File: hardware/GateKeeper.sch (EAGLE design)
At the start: 26 parts, among them K1 G3VM-351A, K2 G3VM-351A, U1 WEMOS-C3-PICO

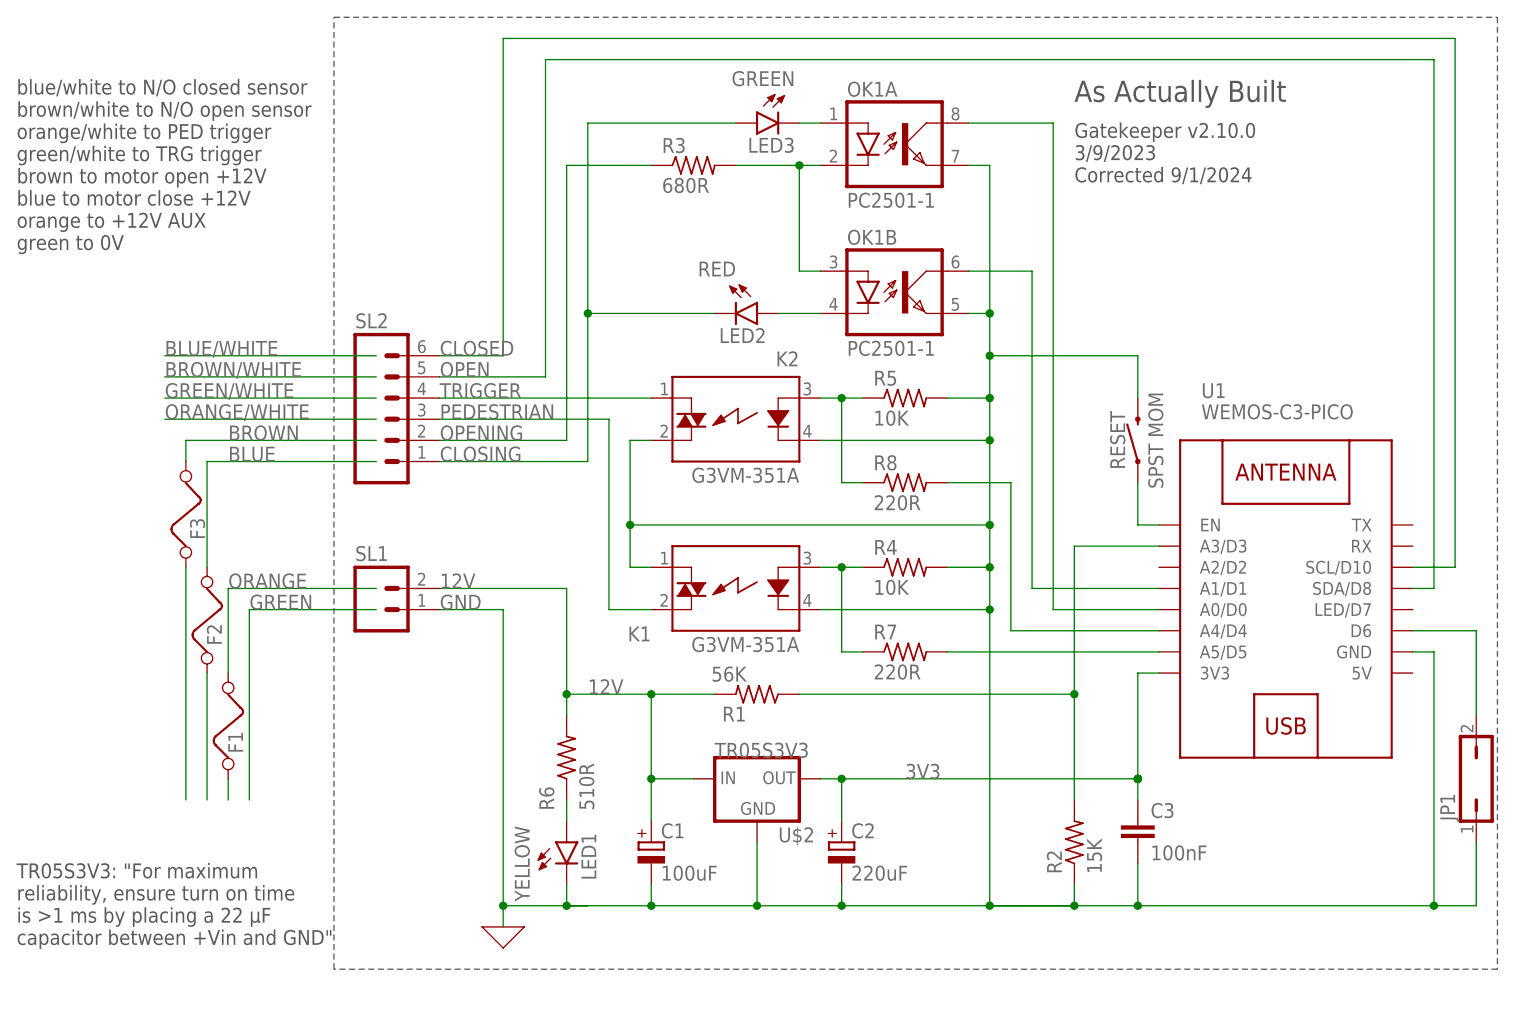
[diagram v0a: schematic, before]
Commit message: Update repository to hardware version 4.6.
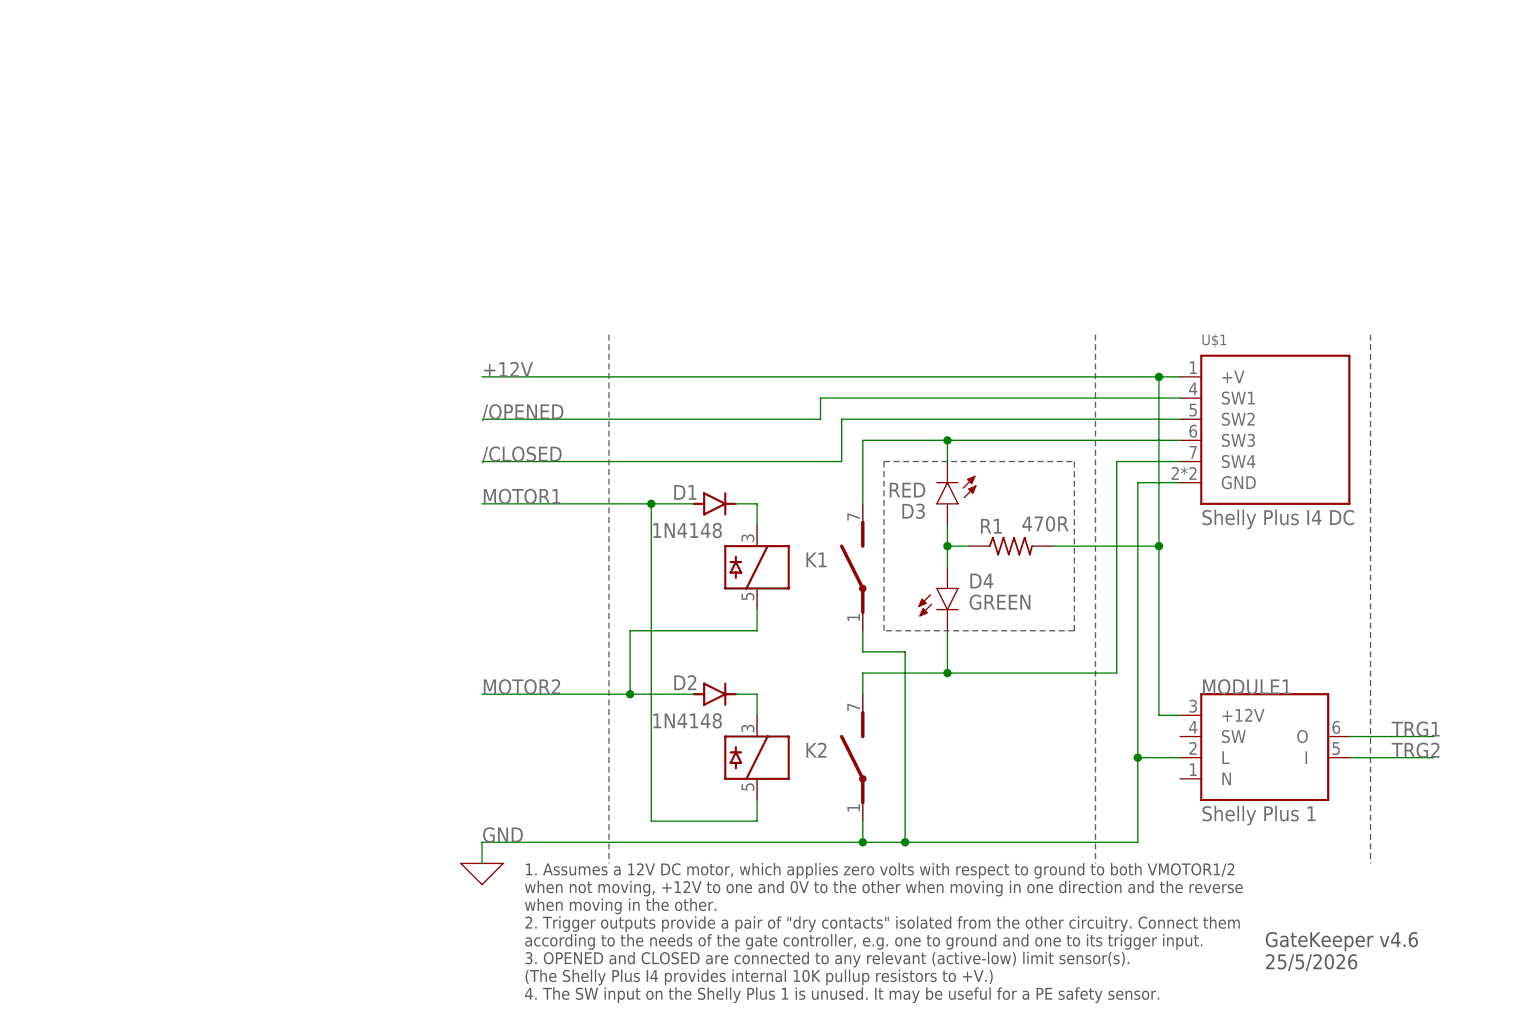
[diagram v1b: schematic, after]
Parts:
- removed C1: 100uF, rcl:CPOL-EUE2.5-5
- removed C2: 220uF, rcl:CPOL-EUE2.5-5
- removed C3: 100nF, capacitor-wima:C2.5/2
- removed F1, F2, F3: (no value), special:FUSE
- removed JP1: (no value), jumper:JP1Q
- removed LED1: YELLOW, led:LED5MM
- removed LED2: RED, led:LED5MM
- removed LED3: GREEN, led:LED5MM
- removed OK1: PC2501-1, optocoupler:PC827
- removed R2: 15K, rcl:R-US_0207/10
- removed R3: 680R, rcl:R-US_0207/10
- removed R4, R5: 10K, rcl:R-US_0207/10
- removed R6: 510R, rcl:R-US_0207/10
- removed R7, R8: 220R, rcl:R-US_0207/10
- removed RESET: SPST MOM, SparkFun-Switches:MOMENTARY-SWITCH-SPST-PTH-6.0MM
- removed SL1: (no value), con-amp-quick:M02
- removed SL2: (no value), con-amp-quick:M06
- removed U$2: TR05S3V3, SparkFun-IC-Power:V_REG_LD1117VXX
- removed U1: WEMOS-C3-PICO, Modules:WEMOS-C3-PICOWEMOS-C3-PICO
- added D1, D2: 1N4148, diode:1N4148DO35-7
- added D3: RED, Opto-Electronic:LED_RADIALRED
- added D4: GREEN, Opto-Electronic:LED_RADIALRED
- added MODULE1: SHELLY_PLUS_1, Shelly:SHELLY_PLUS_1
- added U$1: SHELLY_PLUS_I4_DC, Shelly:SHELLY_PLUS_I4_DC
- K1, K2: value G3VM-351A -> 35701331; device relay:S202SE1 -> relay:35701331
- R1: value 56K -> 470R; device rcl:R-US_0207/10 -> rcl:R-US_0204/2V
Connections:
- removed net 12V: C1.+, R1.2, R6.2, SL1.2, U$2.IN
- removed net 3V3: C2.+, C3.1, U$2.OUT, U1.3V3
- removed net BLUE: F2.2
- removed net BROWN: F3.2
- removed net CLOSED: SL2.6, U1.SCL/D10
- removed net CLOSING: LED2.C, LED3.A, SL2.1
- removed net N$11: F3.1
- removed net N$12: RESET.1, U1.EN
- removed net N$13: JP1.2, U1.D6
- removed net N$14: R8.2, U1.A4/D4
- removed net N$16: K1.A, R4.1, R7.1
- removed net N$21: OK1A.C, OK1B.A, R3.2
- removed net N$4: LED3.C, OK1A.A
- removed net N$6: OK1A.COL, U1.A0/D0
- removed net N$7: K2.A, R5.1, R8.1
- removed net N$8: F2.1
- removed net N$9: LED1.A, R6.1
- removed net OPEN: SL2.5, U1.SDA/D8
- removed net OPENING: R3.1, SL2.2
- removed net ORANGE: F1.2
- removed net PEDESTRIAN: K1.DS2, SL2.3
- removed net TRIGGER: K2.DS1, SL2.4
- new net +12V: MODULE1.+12V, R1.2, U$1.+V
- new net /CLOSED: U$1.SW2
- new net /OPENED: U$1.SW1
- new net MOTOR1: D1.A, K21.5
- new net MOTOR2: D2.A, K11.5
- new net TRG1: MODULE1.O
- new net TRG2: MODULE1.I
- net GND: now also K12.P, K22.P, MODULE1.L, U$1.GND; no longer C1.-, C2.-, C3.2, JP1.1, K1.DS1, K1.K, K2.DS2, K2.K, LED1.C, OK1A.EMIT, OK1B.EMIT, R2.1, R4.2, R5.2, RESET.2, SL1.1, U$2.GND, U1.GND
- net N$1: now also D1.C, K11.3; no longer LED2.A, OK1B.C
- net N$10: now also D3.C, K12.S, U$1.SW3; no longer R1.1, R2.2, U1.A3/D3
- net N$2: now also D2.C, K21.3; no longer R7.2, U1.A5/D5
- net N$3: now also D3.A, D4.A, R1.1; no longer OK1B.COL, U1.A1/D1
- net N$5: now also D4.C, K22.S, U$1.SW4; no longer F1.1
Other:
- note added: "1. Assumes a 12V DC motor, which applies zero volts with respect to ground to both VMOTOR1/2 when not moving, +12V to one and 0V to the other when moving in one direction and the reverse when moving in the other. 2. Trigger outputs provide a pair of "dry contacts" isolated from the other circuitry. Connect them according to the needs of the gate controller, e.g. one to ground and one to its trigg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"
- note added: "GateKeeper v4.6 25/5/2026"
- note removed: "As Actually Built"
- note removed: "Gatekeeper v2.10.0 3/9/2023 Corrected 9/1/2024"
- note removed: "TR05S3V3: "For maximum reliability, ensure turn on time is >1 ms by placing a 22 μF capacitor between +Vin and GND""
- note removed: "blue/white to N/O closed sensor brown/white to N/O open sensor orange/white to PED trigger green/white to TRG trigger brown to motor open +12V blue to motor close +12V orange to +12V AUX green to 0V"
- moved on the sheet: R1
